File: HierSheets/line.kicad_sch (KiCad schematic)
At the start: 72 parts, among them Q10 SFH309, Q11 SFH309, Q12 SFH309, Q17 SFH309, Q18 SFH309, Q19 SFH309, Q20 SFH309, Q21 SFH309, Q22 SFH309, Q23 SFH309, Q24 SFH309, Q25 SFH309, Q26 SFH309, Q27 SFH309, Q28 SFH309, Q9 SFH309, U13 ADS1115IDGS, U14 ADS1115IDGS, U15 ADS1115IDGS, U16 ADS1115IDGS

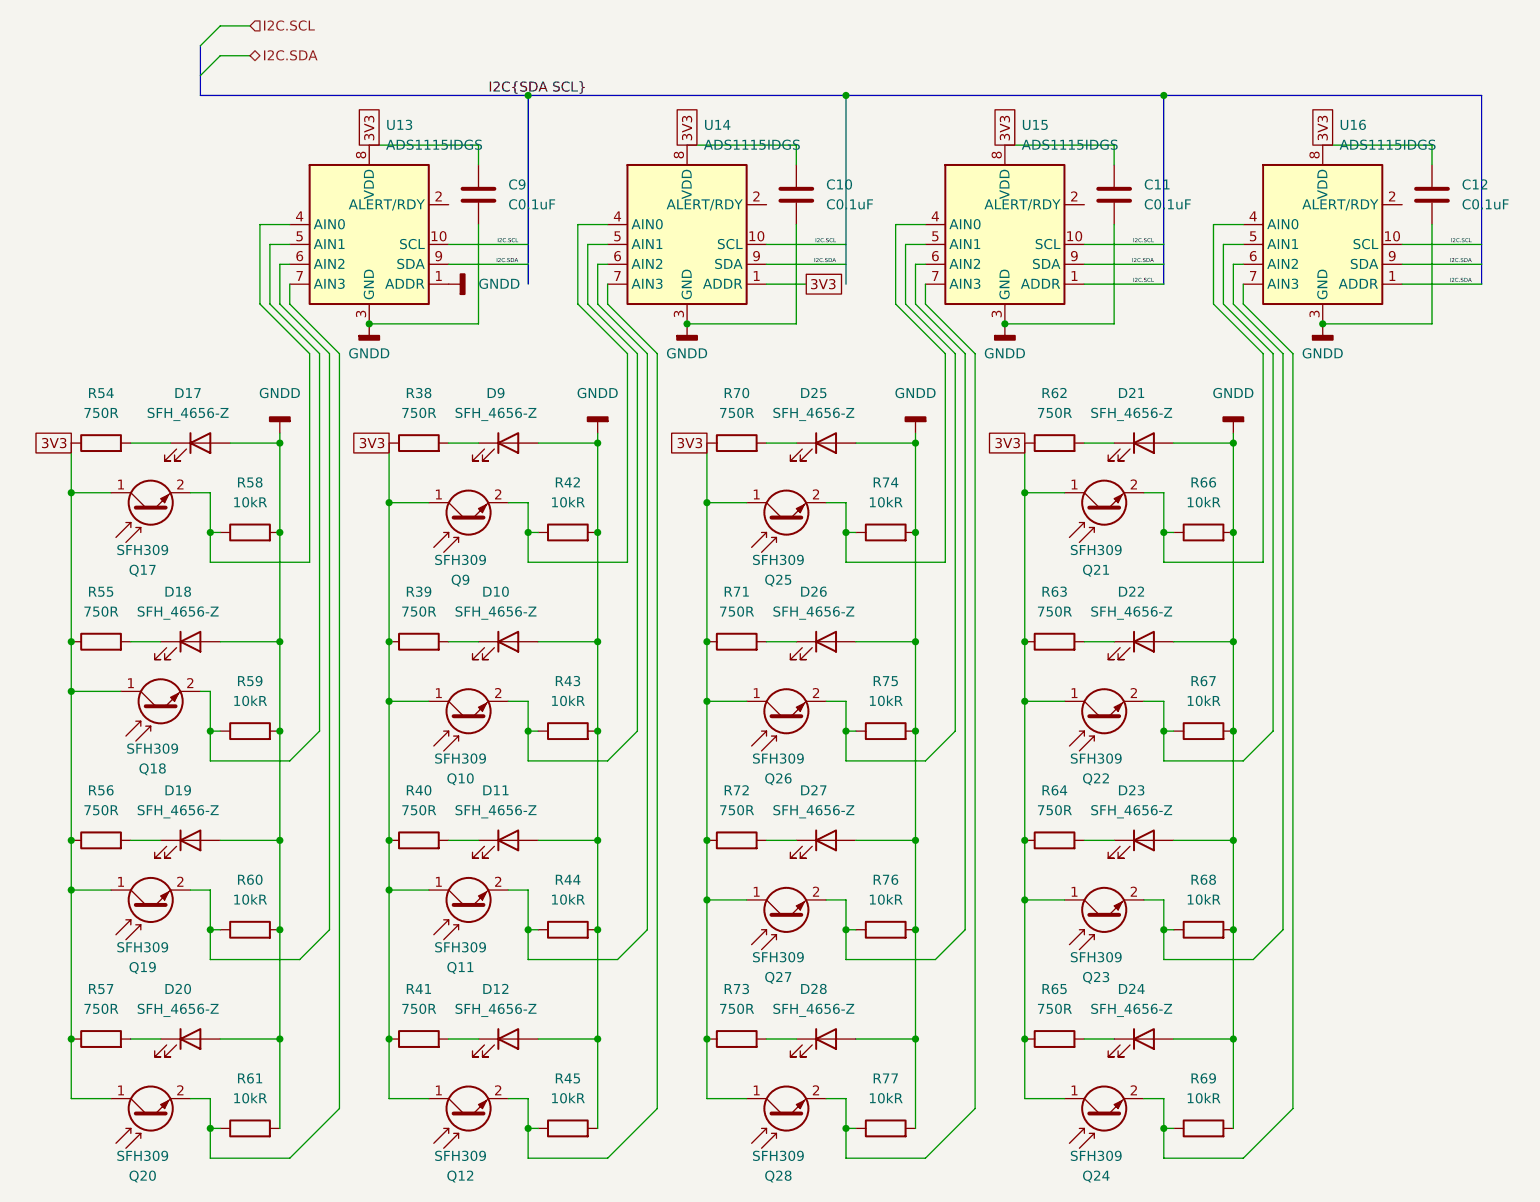
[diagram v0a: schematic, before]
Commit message: aaa
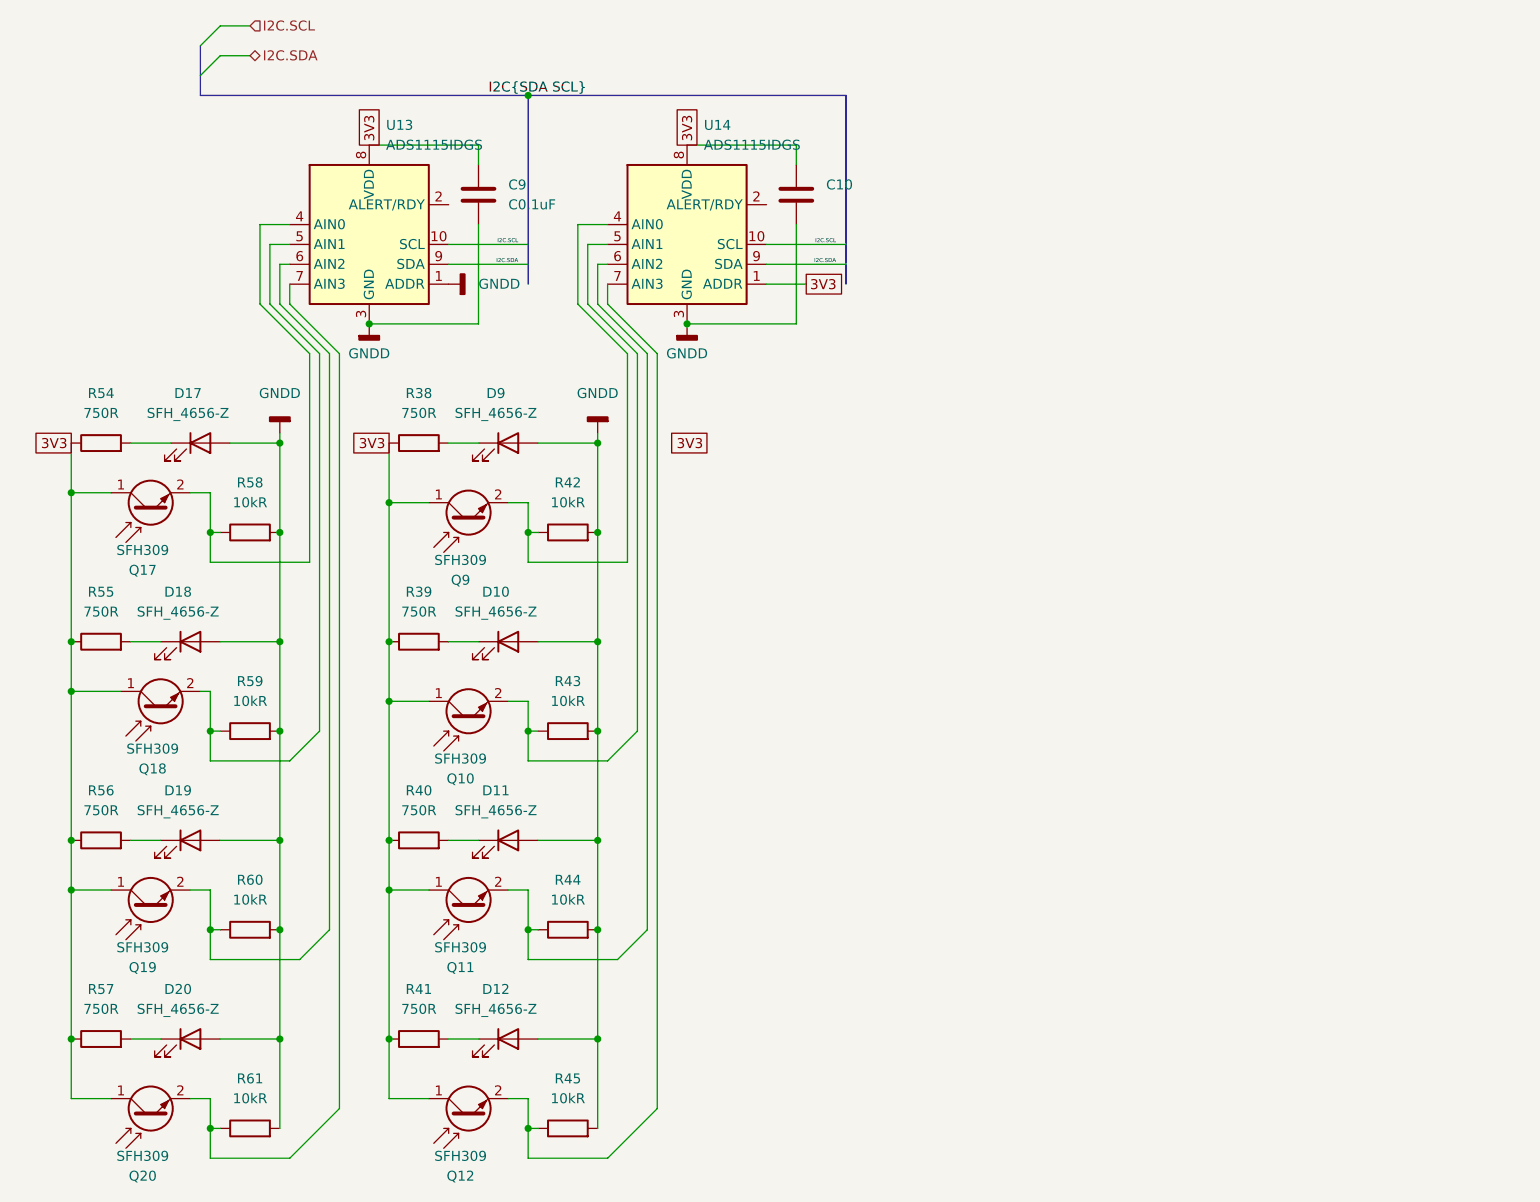
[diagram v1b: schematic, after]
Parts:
- removed C11, C12: C0.1uF, symbol Device:C
- removed D21, D22, D23, D24, D25, D26, D27, D28: SFH_4656-Z, symbol Device:LED
- removed Q21, Q22, Q23, Q24, Q25, Q26, Q27, Q28: SFH309, LED_THT:LED_D3.0mm_Clear, symbol Sensor_Optical:SFH309
- removed R62, R63, R64, R65, R70, R71, R72, R73: 750R, symbol Device:R
- removed R66, R67, R68, R69, R74, R75, R76, R77: 10kR, symbol Device:R
- removed U15, U16: ADS1115IDGS, Package_SO:TSSOP-10_3x3mm_P0.5mm, symbol Analog_ADC:ADS1115IDGS
